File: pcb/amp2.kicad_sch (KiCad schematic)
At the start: 14 parts, among them Q3 BFP640

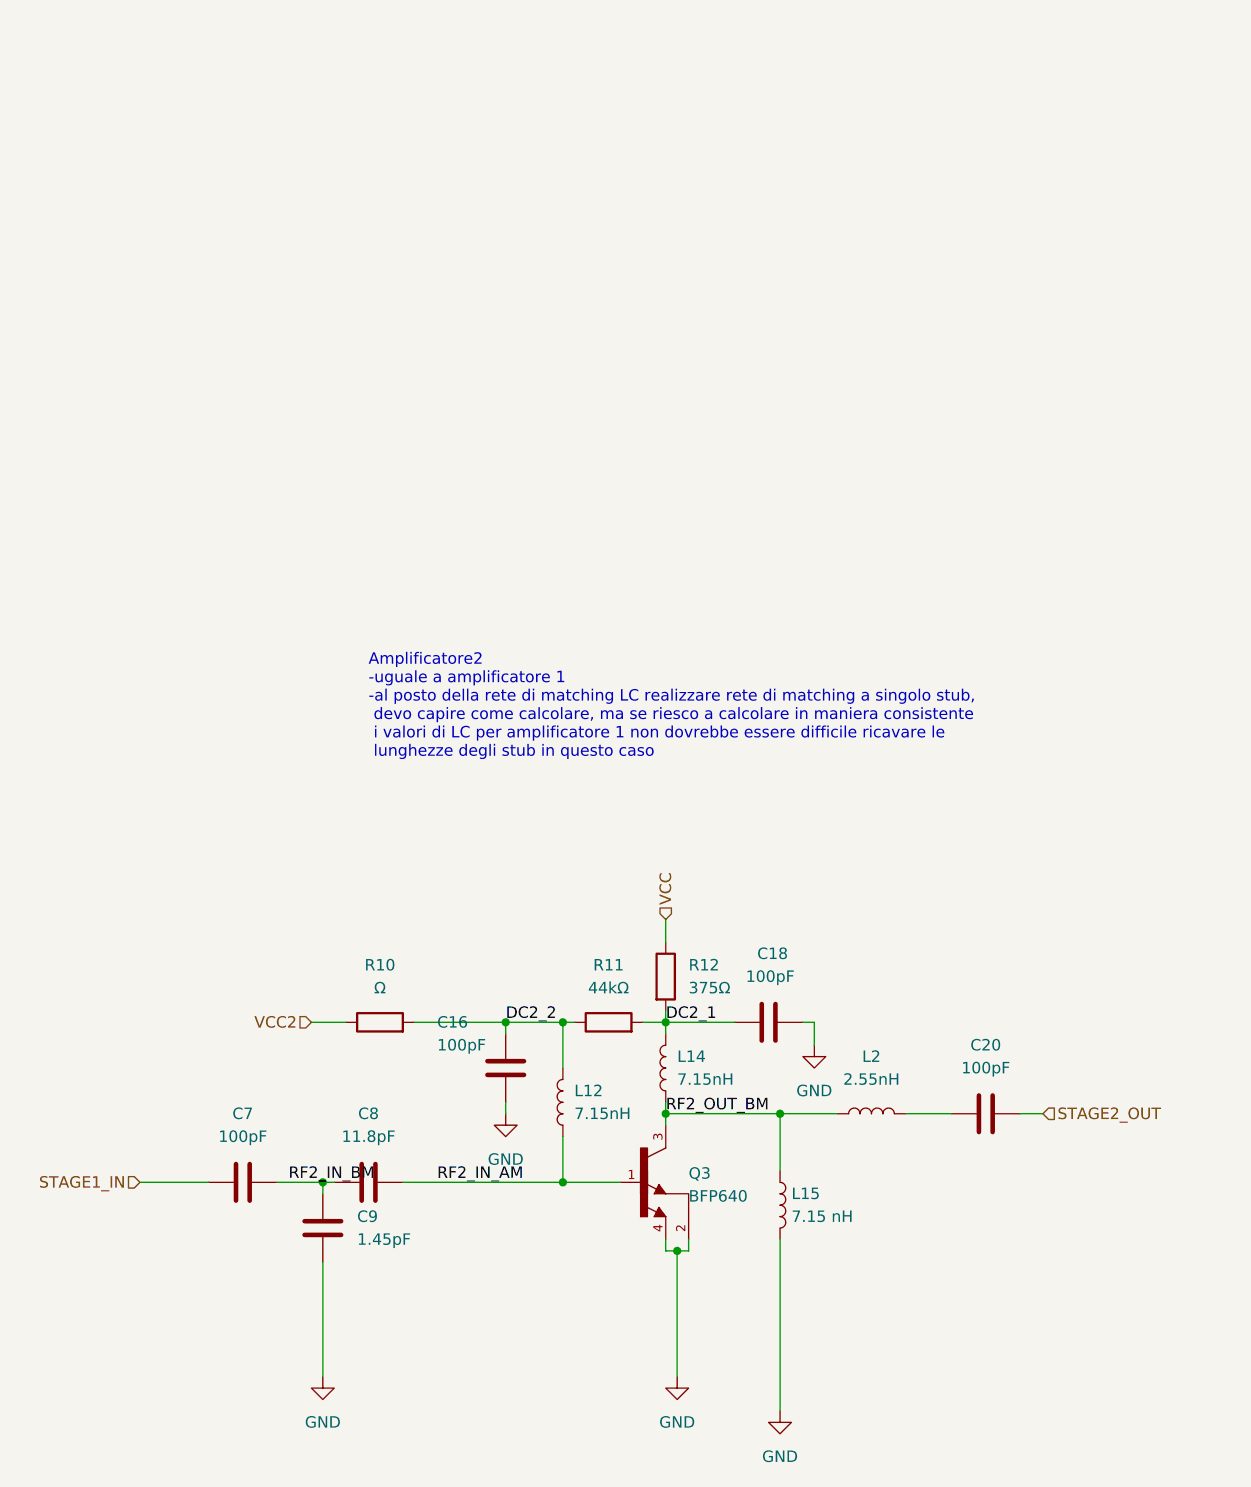
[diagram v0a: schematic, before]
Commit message: graduated
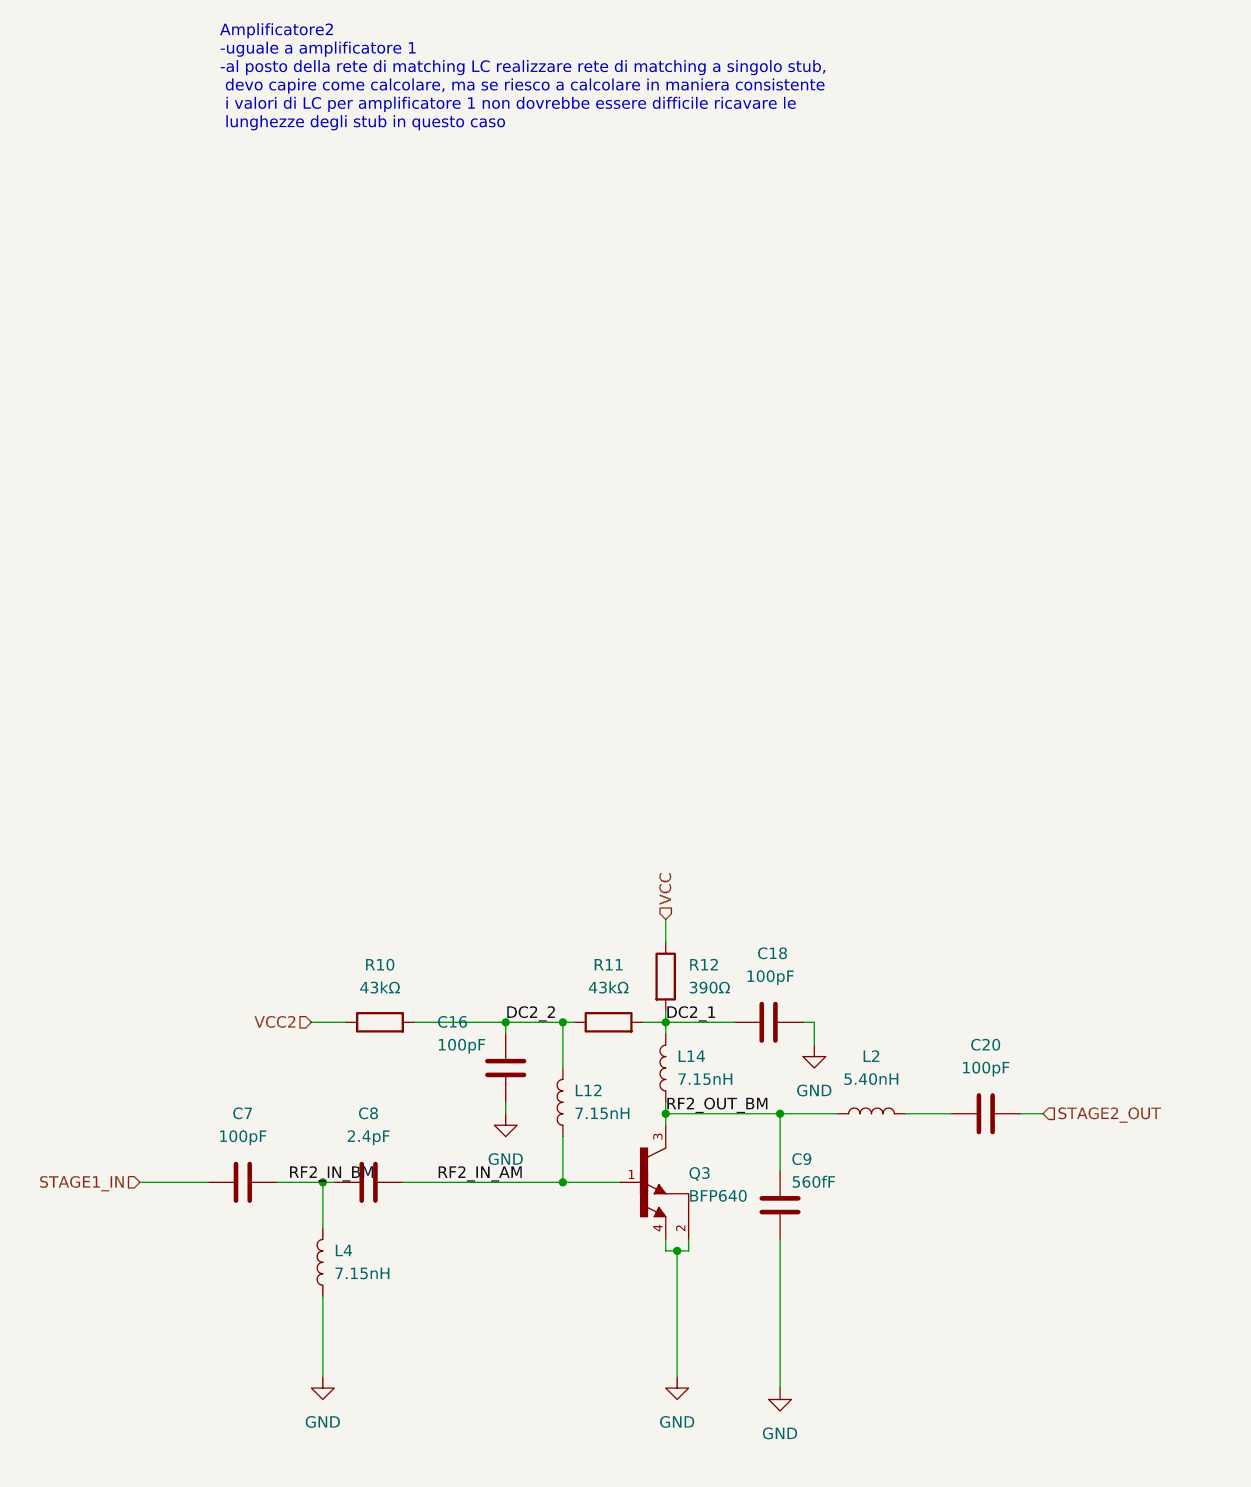
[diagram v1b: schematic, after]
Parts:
- removed L15: 7.15 nH, Nicobigio01:Coilcraft_mod, symbol Device:L
- added L4: 7.15nH, Nicobigio01:Coilcraft_1606-xxLx, symbol Device:L
- C8: value 11.8pF -> 2.4pF
- C9: value 1.45pF -> 560fF
- L2: value 2.55nH -> 5.40nH
- R10: value Ω -> 43kΩ
- R11: value 44kΩ -> 43kΩ
- R12: value 375Ω -> 390Ω
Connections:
- net GND: now also L4.1
- net RF2_IN_BM: now also L4.2; no longer C9.1
- net RF2_OUT_BM: now also C9.1
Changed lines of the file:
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@@
     (stroke (width 0) (type default))
   )
-  (wire (pts (xy 170.18 97.79) (xy 170.18 116.84))
+  (wire (pts (xy 170.18 97.79) (xy 170.18 114.3))
     (stroke (width 0) (type default))
   )
@@
     (stroke (width 0) (type default))
   )
-  (wire (pts (xy 119.38 100.33) (xy 119.38 113.03))
+  (wire (pts (xy 119.38 104.14) (xy 119.38 113.03))
     (stroke (width 0) (type default))
   )
@@
     (stroke (width 0) (type default))
   )
-  (wire (pts (xy 119.38 92.71) (xy 119.38 91.44))
+  (wire (pts (xy 119.38 96.52) (xy 119.38 91.44))
     (stroke (width 0) (type default))
   )
@@
   )
   (text "Amplificatore2\n-uguale a amplificatore 1\n-al posto della rete di matching LC realizzare rete di matching a singolo stub,\n devo capire come calcolare, ma se riesco a calcolare in maniera consistente\n i valori di LC per amplificatore 1 non dovrebbe essere difficile ricavare le\n lunghezze degli stub in questo caso"
-    (at 124.46 44.45 0)
+    (at 107.95 -25.4 0)
     (effects (font (size 1.27 1.27)) (justify left bottom))
   )
@@
     (effects (font (size 1.27 1.27)) (justify left))
   )
-  (symbol (lib_id "Device:L") (at 170.18 93.98 0) (unit 1)
-    (in_bom yes) (on_board yes) (dnp no) (fields_autoplaced)
-    (property "Reference" "L15" (at 171.45 92.7099 0)
-      (effects (font (size 1.27 1.27)) (justify left))
-    )
-    (property "Value" "7.15 nH" (at 171.45 95.2499 0)
-      (effects (font (size 1.27 1.27)) (justify left))
-    )
-    (property "Footprint" "Nicobigio01:Coilcraft_mod" (at 170.18 93.98 0)
-      (effects (font (size 1.27 1.27)) hide)
-    )
-    (property "Datasheet" "~" (at 170.18 93.98 0)
-      (effects (font (size 1.27 1.27)) hide)
-    )
-    (pin "1")
-    (pin "2")
-    (instances
-      (project "tesina"
-        (path "/e748d439-ff35-430a-8909-e8d82d6fa64c/4e3d076a-abc7-4ccc-a891-541b92d429fd"
-          (reference "L15") (unit 1)
-        )
-      )
-    )
-  )
   (symbol (lib_id "Device:R") (at 125.73 73.66 90) (unit 1)
     (in_bom yes) (on_board yes) (dnp no) (fields_autoplaced)
@@
       (effects (font (size 1.27 1.27)))
     )
-    (property "Value" "Ω" (at 125.73 69.85 90)
+    (property "Value" "43kΩ" (at 125.73 69.85 90)
       (effects (font (size 1.27 1.27)))
     )
@@
       (effects (font (size 1.27 1.27)))
     )
-    (property "Value" "11.8pF" (at 124.46 86.36 90)
+    (property "Value" "2.4pF" (at 124.46 86.36 90)
       (effects (font (size 1.27 1.27)))
     )
@@
         (path "/e748d439-ff35-430a-8909-e8d82d6fa64c/4e3d076a-abc7-4ccc-a891-541b92d429fd"
           (reference "#PWR0129") (unit 1)
+        )
+      )
+    )
+  )
+  (symbol (lib_id "Device:C") (at 170.18 93.98 0) (mirror y) (unit 1)
+    (in_bom yes) (on_board yes) (dnp no)
+    (property "Reference" "C9" (at 171.45 88.9 0)
+      (effects (font (size 1.27 1.27)) (justify right))
+    )
+    (property "Value" "560fF" (at 171.45 91.44 0)
+      (effects (font (size 1.27 1.27)) (justify right))
+    )
+    (property "Footprint" "Capacitor_SMD:C_0603_1608Metric" (at 169.2148 97.79 0)
+      (effects (font (size 1.27 1.27)) hide)
+    )
+    (property "Datasheet" "~" (at 170.18 93.98 0)
+      (effects (font (size 1.27 1.27)) hide)
+    )
+    (pin "1")
+    (pin "2")
+    (instances
+      (project "tesina"
+        (path "/e748d439-ff35-430a-8909-e8d82d6fa64c/4e3d076a-abc7-4ccc-a891-541b92d429fd"
+          (reference "C9") (unit 1)
         )
       )
@@
       (effects (font (size 1.27 1.27)) (justify left))
     )
-    (property "Value" "375Ω" (at 160.02 69.8499 0)
+    (property "Value" "390Ω" (at 160.02 69.8499 0)
       (effects (font (size 1.27 1.27)) (justify left))
     )
@@
       (effects (font (size 1.27 1.27)))
     )
-    (property "Value" "2.55nH" (at 180.34 80.01 90)
+    (property "Value" "5.40nH" (at 180.34 80.01 90)
       (effects (font (size 1.27 1.27)))
     )
@@
       (effects (font (size 1.27 1.27)))
     )
-    (property "Value" "44kΩ" (at 151.13 69.85 90)
+    (property "Value" "43kΩ" (at 151.13 69.85 90)
       (effects (font (size 1.27 1.27)))
     )
@@
     )
   )
-  (symbol (lib_id "Device:C") (at 119.38 96.52 0) (unit 1)
-    (in_bom yes) (on_board yes) (dnp no) (fields_autoplaced)
-    (property "Reference" "C9" (at 123.19 95.2499 0)
-      (effects (font (size 1.27 1.27)) (justify left))
-    )
-    (property "Value" "1.45pF" (at 123.19 97.7899 0)
-      (effects (font (size 1.27 1.27)) (justify left))
-    )
-    (property "Footprint" "Capacitor_SMD:C_0603_1608Metric" (at 120.3452 100.33 0)
-      (effects (font (size 1.27 1.27)) hide)
-    )
-    (property "Datasheet" "~" (at 119.38 96.52 0)
-      (effects (font (size 1.27 1.27)) hide)
-    )
-    (pin "1")
-    (pin "2")
-    (instances
-      (project "tesina"
-        (path "/e748d439-ff35-430a-8909-e8d82d6fa64c/4e3d076a-abc7-4ccc-a891-541b92d429fd"
-          (reference "C9") (unit 1)
-        )
-      )
-    )
-  )
-  (symbol (lib_id "power:GND") (at 170.18 116.84 0) (unit 1)
-    (in_bom yes) (on_board yes) (dnp no) (fields_autoplaced)
-    (property "Reference" "#PWR0128" (at 170.18 123.19 0)
-      (effects (font (size 1.27 1.27)) hide)
-    )
-    (property "Value" "GND" (at 170.18 121.92 0)
-      (effects (font (size 1.27 1.27)))
-    )
-    (property "Footprint" "" (at 170.18 116.84 0)
-      (effects (font (size 1.27 1.27)) hide)
-    )
-    (property "Datasheet" "" (at 170.18 116.84 0)
-      (effects (font (size 1.27 1.27)) hide)
-    )
+  (symbol (lib_id "Device:L") (at 119.38 100.33 180) (unit 1)
+    (in_bom yes) (on_board yes) (dnp no) (fields_autoplaced)
+    (property "Reference" "L4" (at 120.65 99.0599 0)
+      (effects (font (size 1.27 1.27)) (justify right))
+    )
+    (property "Value" "7.15nH" (at 120.65 101.5999 0)
+      (effects (font (size 1.27 1.27)) (justify right))
+    )
+    (property "Footprint" "Nicobigio01:Coilcraft_1606-xxLx" (at 119.38 100.33 0)
+      (effects (font (size 1.27 1.27)) hide)
+    )
+    (property "Datasheet" "~" (at 119.38 100.33 0)
+      (effects (font (size 1.27 1.27)) hide)
+    )
+    (pin "1")
+    (pin "2")
+    (instances
+      (project "tesina"
+        (path "/e748d439-ff35-430a-8909-e8d82d6fa64c/4e3d076a-abc7-4ccc-a891-541b92d429fd"
+          (reference "L4") (unit 1)
+        )
+      )
+    )
+  )
+  (symbol (lib_id "power:GND") (at 170.18 114.3 0) (unit 1)
+    (in_bom yes) (on_board yes) (dnp no) (fields_autoplaced)
+    (property "Reference" "#PWR0128" (at 170.18 120.65 0)
+      (effects (font (size 1.27 1.27)) hide)
+    )
+    (property "Value" "GND" (at 170.18 119.38 0)
+      (effects (font (size 1.27 1.27)))
+    )
+    (property "Footprint" "" (at 170.18 114.3 0)
+      (effects (font (size 1.27 1.27)) hide)
+    )
+    (property "Datasheet" "" (at 170.18 114.3 0)
+      (effects (font (size 1.27 1.27)) hide)
+    )
